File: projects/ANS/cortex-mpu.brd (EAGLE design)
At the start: 100 x 80 mm, 71 parts, among them IC1 LM1117MPX-3.3, U1 AT32UC3B164-AUT, Y1 7A-16

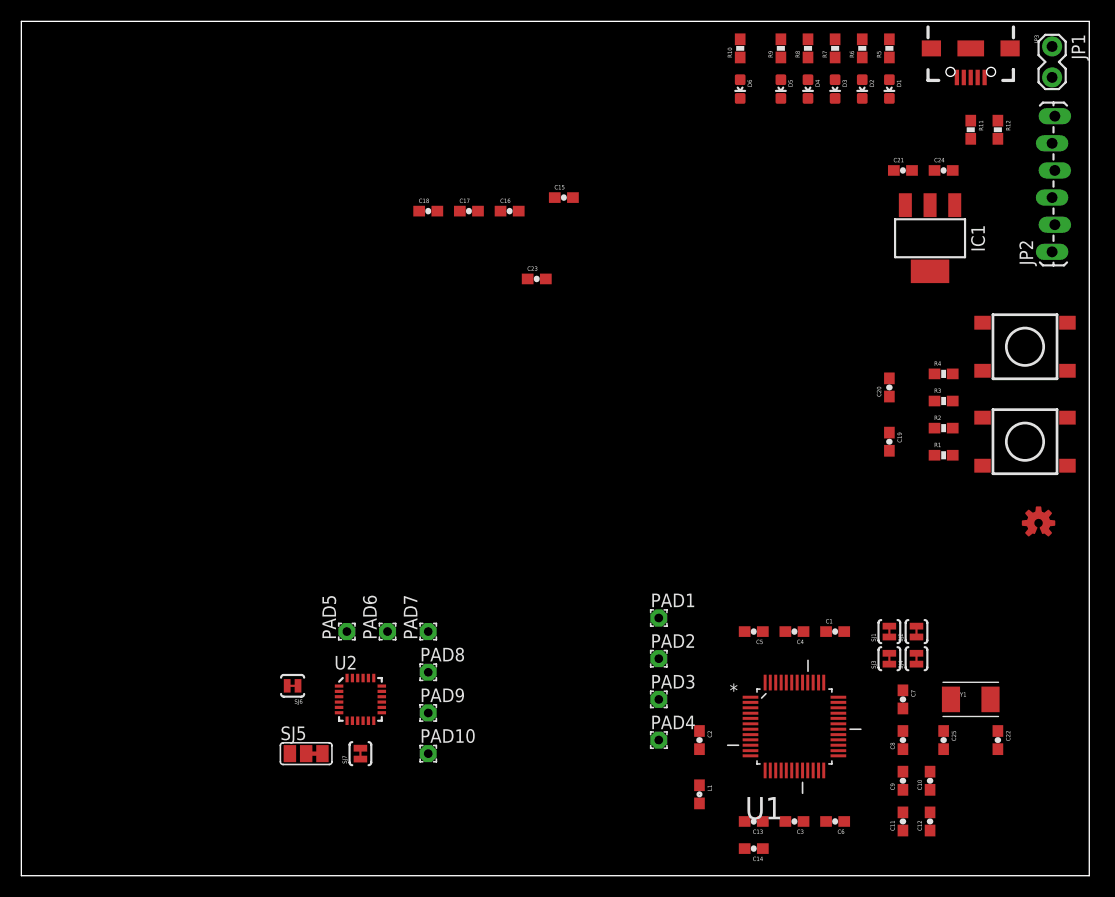
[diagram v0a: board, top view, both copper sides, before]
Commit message: brd
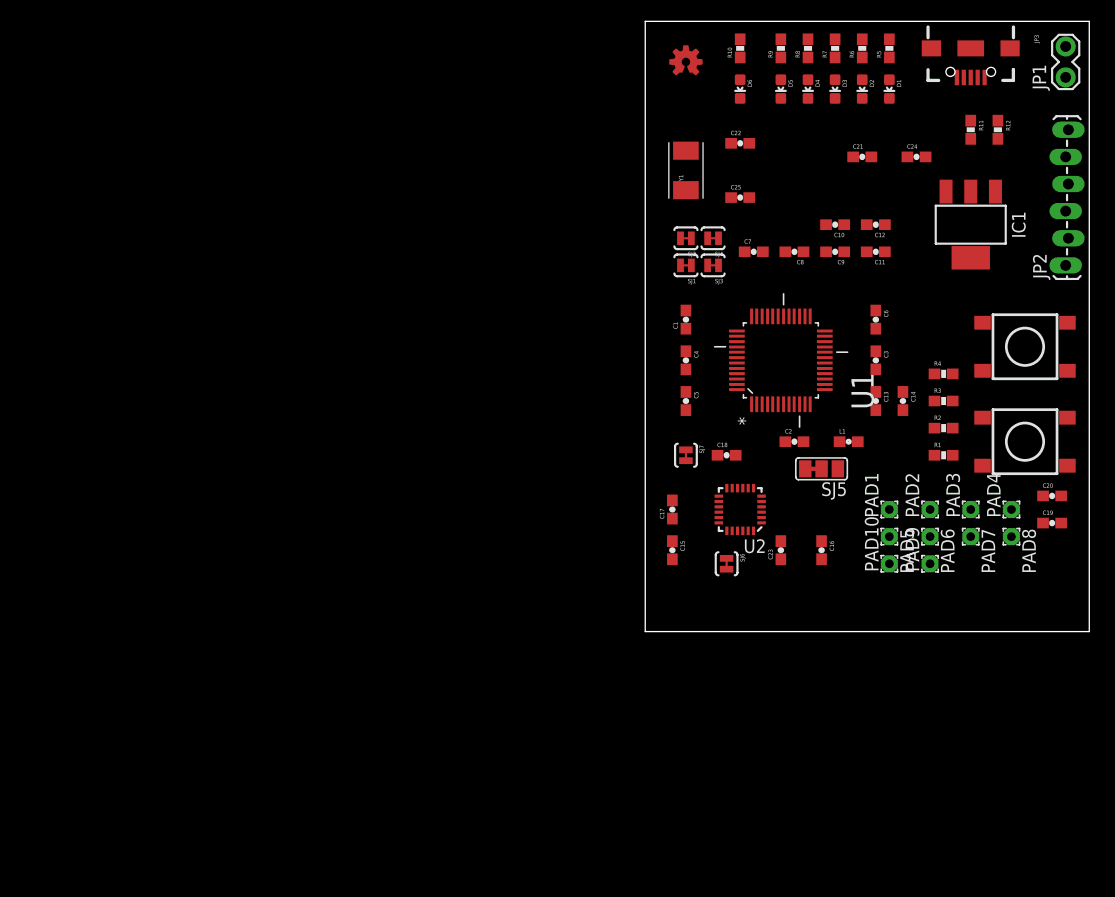
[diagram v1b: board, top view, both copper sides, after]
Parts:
- moved C22 60.9 mm to (67.3, 68.6), turned to 0 degrees
- moved Y1 56.3 mm to (62.2, 66.0), turned to 90 degrees
- moved C12 56.1 mm to (80.0, 61.0), turned to 180 degrees
- moved PAD8 56.1 mm to (92.7, 31.8), turned to 270 degrees
- moved SJ5 55.1 mm to (74.9, 38.1), turned to 180 degrees
- moved LOGO1 54.4 mm to (62.2, 76.2)
- moved C25 54.3 mm to (67.3, 63.5), turned to 0 degrees
- moved C11 53.4 mm to (80.0, 58.4), turned to 180 degrees
- moved C10 52.8 mm to (76.2, 61.0), turned to 180 degrees
- moved PAD6 51.6 mm to (85.1, 31.8), turned to 270 degrees
- moved PAD7 51.6 mm to (88.9, 31.8), turned to 270 degrees
- moved PAD5 51.6 mm to (81.3, 31.8), turned to 270 degrees
- moved C9 49.9 mm to (76.2, 58.4), turned to 180 degrees
- moved PAD9 49.0 mm to (85.1, 29.2), turned to 90 degrees
- moved C6 47.1 mm to (80.0, 52.1), turned to 270 degrees
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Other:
- board size 100 x 80 mm -> 41.6 x 57.1 mm
